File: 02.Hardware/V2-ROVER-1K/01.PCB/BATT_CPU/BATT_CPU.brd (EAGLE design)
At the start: 20.8 x 34.8 mm, 70 parts, among them K2 FLEX12, Q1 BSS84W-7-F, Q2 BSS84W-7-F, Q3 2N7002PW, Q4 2N7002PW, Q5 BSS84W-7-F, U1 ATSAMD21G18_QFN, U3 TPS78230DDCR, U6 MAX9062EUK+T, U8 SN74LVC1G19DBVR, X2 32.768

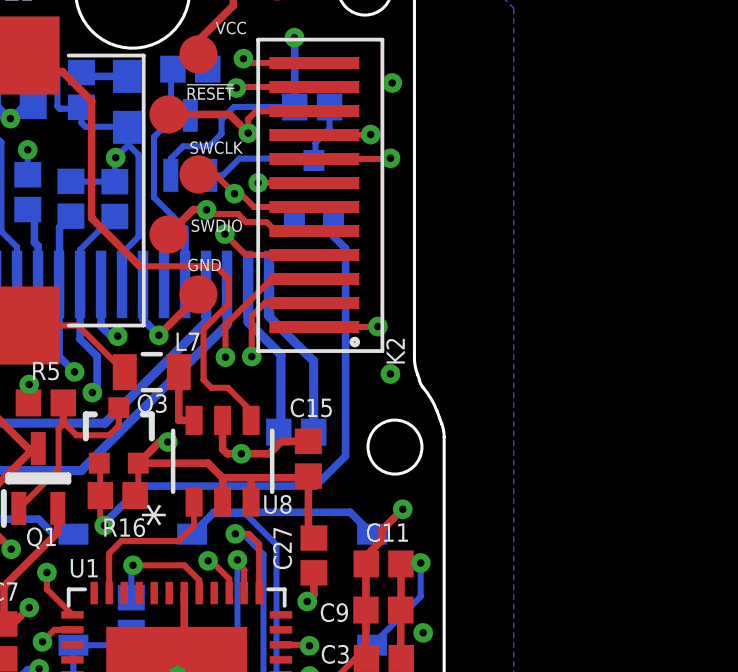
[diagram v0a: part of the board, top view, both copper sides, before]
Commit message: Actualizacion CPU y PROG_BATT
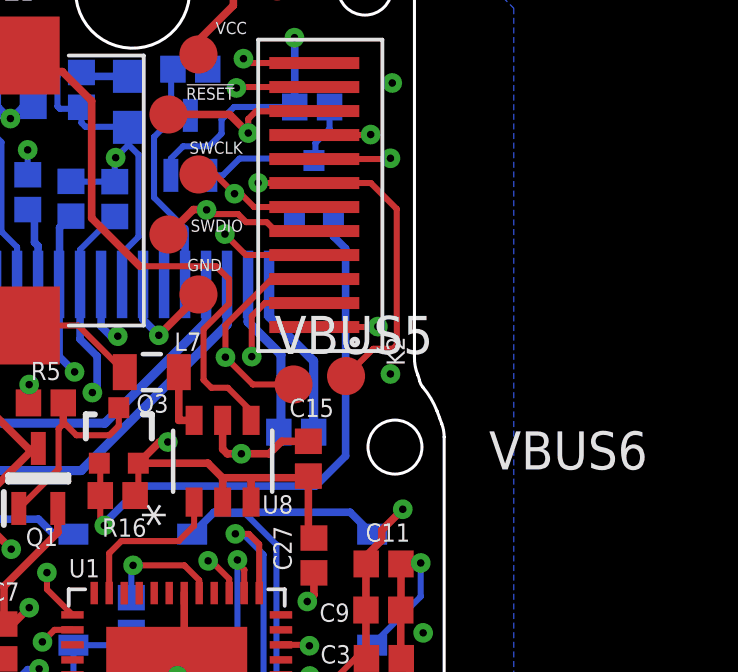
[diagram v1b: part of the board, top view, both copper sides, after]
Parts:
- added VBUS5, VBUS6: TESTPAD_TPSQB1,27, BeagleBone_Blue_R3:TESTPAD_B1,27
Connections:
- net TXO: now also VBUS6.TP
- net VBUS: now also VBUS5.TP
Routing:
- net TXO: track 30.7 -> 40.4 mm
- net VBUS: track 74.7 -> 77.4 mm
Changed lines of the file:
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@@
 <layers>
 <layer number="1" name="Top" color="4" fill="1" visible="yes" active="yes"/>
-<layer number="2" name="Route2" color="11" fill="1" visible="yes" active="yes"/>
+<layer number="2" name="Route2" color="11" fill="1" visible="no" active="yes"/>
 <layer number="3" name="Route3" color="4" fill="3" visible="no" active="no"/>
 <layer number="4" name="Route4" color="1" fill="4" visible="no" active="no"/>
@@
 <layer number="13" name="Route13" color="4" fill="5" visible="no" active="no"/>
 <layer number="14" name="Route14" color="1" fill="6" visible="no" active="no"/>
-<layer number="15" name="GND" color="13" fill="1" visible="yes" active="yes"/>
-<layer number="16" name="Bottom" color="1" fill="1" visible="yes" active="yes"/>
+<layer number="15" name="GND" color="13" fill="1" visible="no" active="yes"/>
+<layer number="16" name="Bottom" color="1" fill="1" visible="no" active="yes"/>
 <layer number="17" name="Pads" color="2" fill="1" visible="yes" active="yes"/>
 <layer number="18" name="Vias" color="2" fill="1" visible="yes" active="yes"/>
 <layer number="19" name="Unrouted" color="6" fill="1" visible="yes" active="yes"/>
 <layer number="20" name="Dimension" color="15" fill="1" visible="yes" active="yes"/>
-<layer number="21" name="tPlace" color="14" fill="1" visible="no" active="yes"/>
-<layer number="22" name="bPlace" color="13" fill="1" visible="yes" active="yes"/>
-<layer number="23" name="tOrigins" color="14" fill="1" visible="no" active="yes"/>
-<layer number="24" name="bOrigins" color="13" fill="1" visible="yes" active="yes"/>
-<layer number="25" name="tNames" color="7" fill="1" visible="no" active="yes"/>
-<layer number="26" name="bNames" color="7" fill="1" visible="yes" active="yes"/>
+<layer number="21" name="tPlace" color="14" fill="1" visible="yes" active="yes"/>
+<layer number="22" name="bPlace" color="13" fill="1" visible="no" active="yes"/>
+<layer number="23" name="tOrigins" color="14" fill="1" visible="yes" active="yes"/>
+<layer number="24" name="bOrigins" color="13" fill="1" visible="no" active="yes"/>
+<layer number="25" name="tNames" color="7" fill="1" visible="yes" active="yes"/>
+<layer number="26" name="bNames" color="7" fill="1" visible="no" active="yes"/>
 <layer number="27" name="tValues" color="7" fill="1" visible="no" active="yes"/>
 <layer number="28" name="bValues" color="7" fill="1" visible="no" active="yes"/>
@@
 <layer number="37" name="tTest" color="7" fill="1" visible="no" active="yes"/>
 <layer number="38" name="bTest" color="7" fill="1" visible="no" active="yes"/>
-<layer number="39" name="tKeepout" color="4" fill="11" visible="no" active="yes"/>
-<layer number="40" name="bKeepout" color="1" fill="11" visible="yes" active="yes"/>
-<layer number="41" name="tRestrict" color="4" fill="10" visible="no" active="yes"/>
-<layer number="42" name="bRestrict" color="1" fill="10" visible="yes" active="yes"/>
+<layer number="39" name="tKeepout" color="4" fill="11" visible="yes" active="yes"/>
+<layer number="40" name="bKeepout" color="1" fill="11" visible="no" active="yes"/>
+<layer number="41" name="tRestrict" color="4" fill="10" visible="yes" active="yes"/>
+<layer number="42" name="bRestrict" color="1" fill="10" visible="no" active="yes"/>
 <layer number="43" name="vRestrict" color="2" fill="10" visible="no" active="yes"/>
 <layer number="44" name="Drills" color="7" fill="1" visible="no" active="yes"/>
@@
 <layer number="49" name="Reference" color="7" fill="1" visible="no" active="yes"/>
 <layer number="50" name="dxf" color="7" fill="1" visible="no" active="yes"/>
-<layer number="51" name="tDocu" color="7" fill="1" visible="no" active="yes"/>
-<layer number="52" name="bDocu" color="7" fill="1" visible="yes" active="yes"/>
+<layer number="51" name="tDocu" color="7" fill="1" visible="yes" active="yes"/>
+<layer number="52" name="bDocu" color="7" fill="1" visible="no" active="yes"/>
 <layer number="53" name="tGND_GNDA" color="7" fill="9" visible="no" active="no"/>
 <layer number="54" name="bGND_GNDA" color="1" fill="9" visible="no" active="no"/>
@@
 <attribute name="VALUE" value="0.1uF" x="20.48" y="13.87" size="1.27" layer="27" rot="R90"/>
 </element>
+<element name="VBUS5" library="BeagleBone_Blue_R3" package="TESTPAD_B1,27" value="TESTPAD_TPSQB1,27" x="17.26" y="20.84" smashed="yes">
+<attribute name="NAME" x="16.625" y="21.856" size="1.27" layer="25" ratio="10"/>
+<attribute name="TP_SIGNAL_NAME" value="" x="16.625" y="18.935" size="1" layer="37"/>
+<attribute name="VALUE" x="16.625" y="20.078" size="0.0254" layer="27"/>
+</element>
+<element name="VBUS6" library="BeagleBone_Blue_R3" package="TESTPAD_B1,27" value="TESTPAD_TPSQB1,27" x="19.01" y="21.12" smashed="yes">
+<attribute name="NAME" x="23.775" y="18.006" size="1.27" layer="25" ratio="10"/>
+<attribute name="TP_SIGNAL_NAME" value="" x="18.375" y="19.215" size="1" layer="37"/>
+<attribute name="VALUE" x="18.375" y="20.358" size="0.0254" layer="27"/>
+</element>
 </elements>
 <signals>
@@
 <wire x1="6.117" y1="16.557" x2="6.117" y2="16.637" width="0.2032" layer="1"/>
 <wire x1="6.117" y1="16.637" x2="6.287" y2="16.807" width="0.2032" layer="1"/>
+<contactref element="VBUS5" pad="TP"/>
+<wire x1="14.99" y1="21.75" x2="15.9" y2="20.84" width="0.2032" layer="1"/>
+<wire x1="15.9" y1="20.84" x2="17.26" y2="20.84" width="0.2032" layer="1"/>
 </signal>
 <signal name="AREF">
@@
 <wire x1="10.615" y1="6.355" x2="10.615" y2="6.936" width="0.2032" layer="1"/>
 <wire x1="11" y1="5.97" x2="10.615" y2="6.355" width="0.2032" layer="1"/>
+<contactref element="VBUS6" pad="TP"/>
+<wire x1="19.01" y1="21.12" x2="19.92" y2="22.03" width="0.2032" layer="1"/>
+<wire x1="19.92" y1="22.03" x2="20.57" y2="22.03" width="0.2032" layer="1"/>
+<wire x1="20.703" y1="23.0322" x2="20.7" y2="23.0352" width="0.2032" layer="1"/>
+<wire x1="20.57" y1="22.03" x2="20.703" y2="22.163" width="0.2032" layer="1"/>
+<wire x1="20.703" y1="22.163" x2="20.703" y2="23.0322" width="0.2032" layer="1"/>
+<wire x1="19.836" y1="27.554" x2="17.951" y2="27.554" width="0.2032" layer="1"/>
+<wire x1="20.7" y1="23.0352" x2="20.7" y2="26.69" width="0.2032" layer="1"/>
+<wire x1="20.7" y1="26.69" x2="19.836" y2="27.554" width="0.2032" layer="1"/>
 </signal>
 <signal name="VINSENSE">
